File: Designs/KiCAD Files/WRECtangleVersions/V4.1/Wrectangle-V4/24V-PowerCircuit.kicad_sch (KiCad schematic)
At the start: 26 parts, among them M1-24V1 60V, M2-24V1 40V, U7 TPS43060RTER

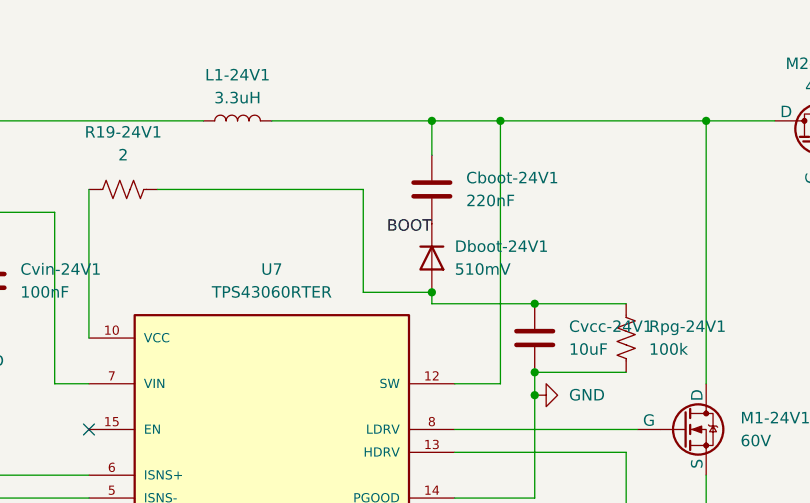
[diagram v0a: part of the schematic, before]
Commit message: Update 24V-PowerCircuit.kicad_sch
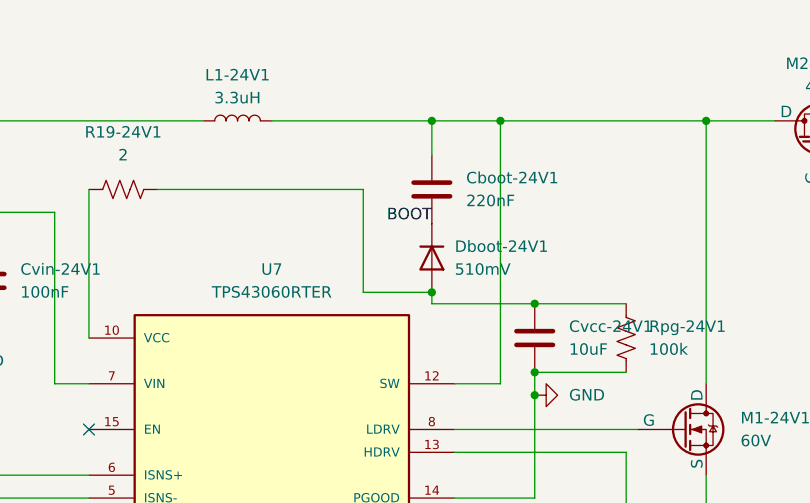
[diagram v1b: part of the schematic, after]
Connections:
- net BOOT: now also Cboot-24V1.1, Dboot-24V1.1 (K)
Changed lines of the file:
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@@
 	)
 	(label "BOOT"
-		(at 181.61 58.42 180)
+		(at 181.61 57.15 180)
 		(effects
 			(font

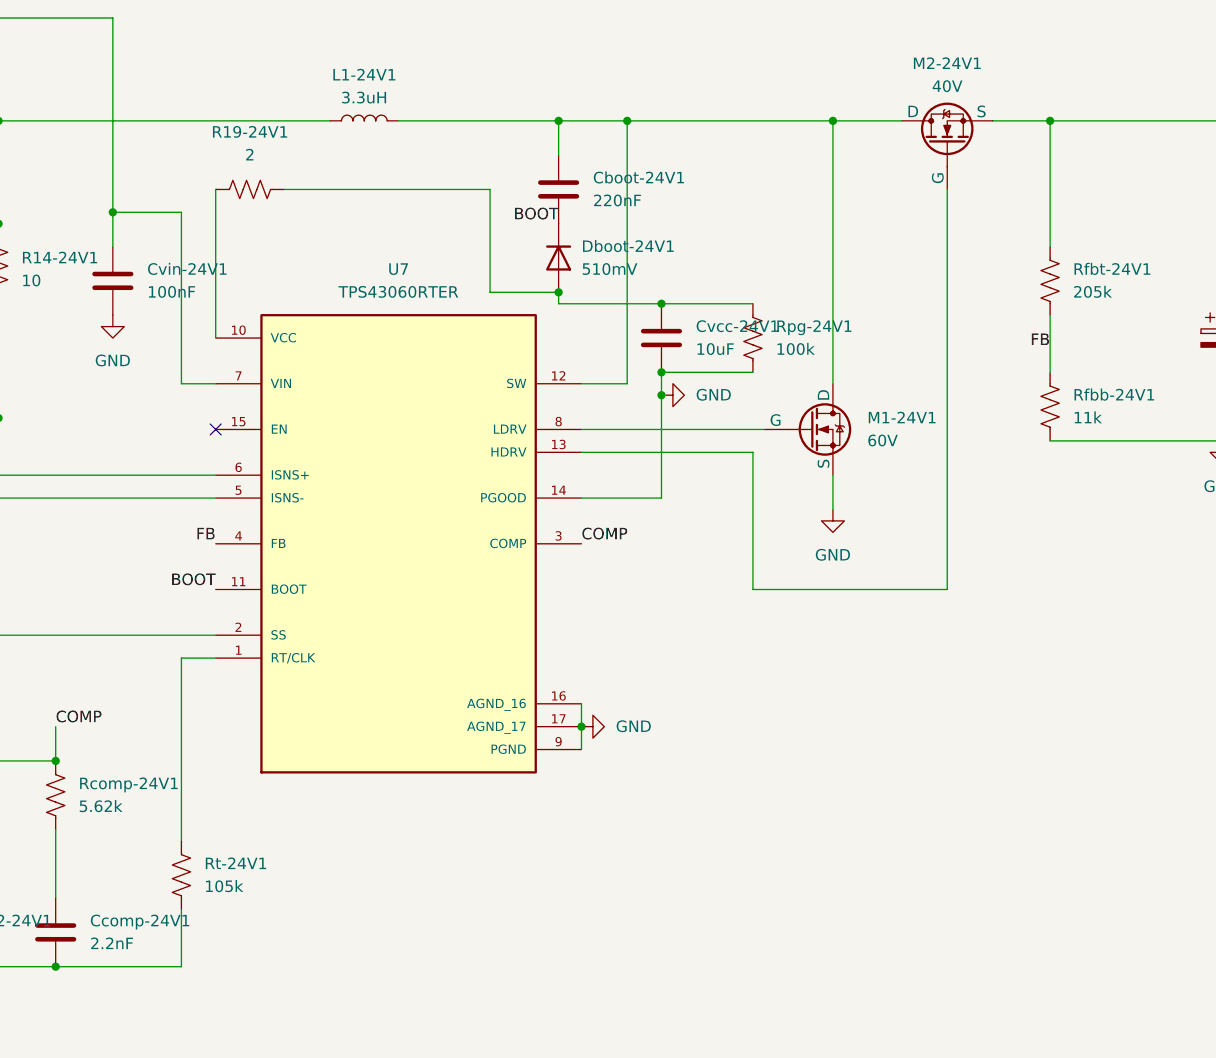
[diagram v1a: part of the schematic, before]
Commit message: Update some schematics (1x)
2-20-26 fixed (#1)
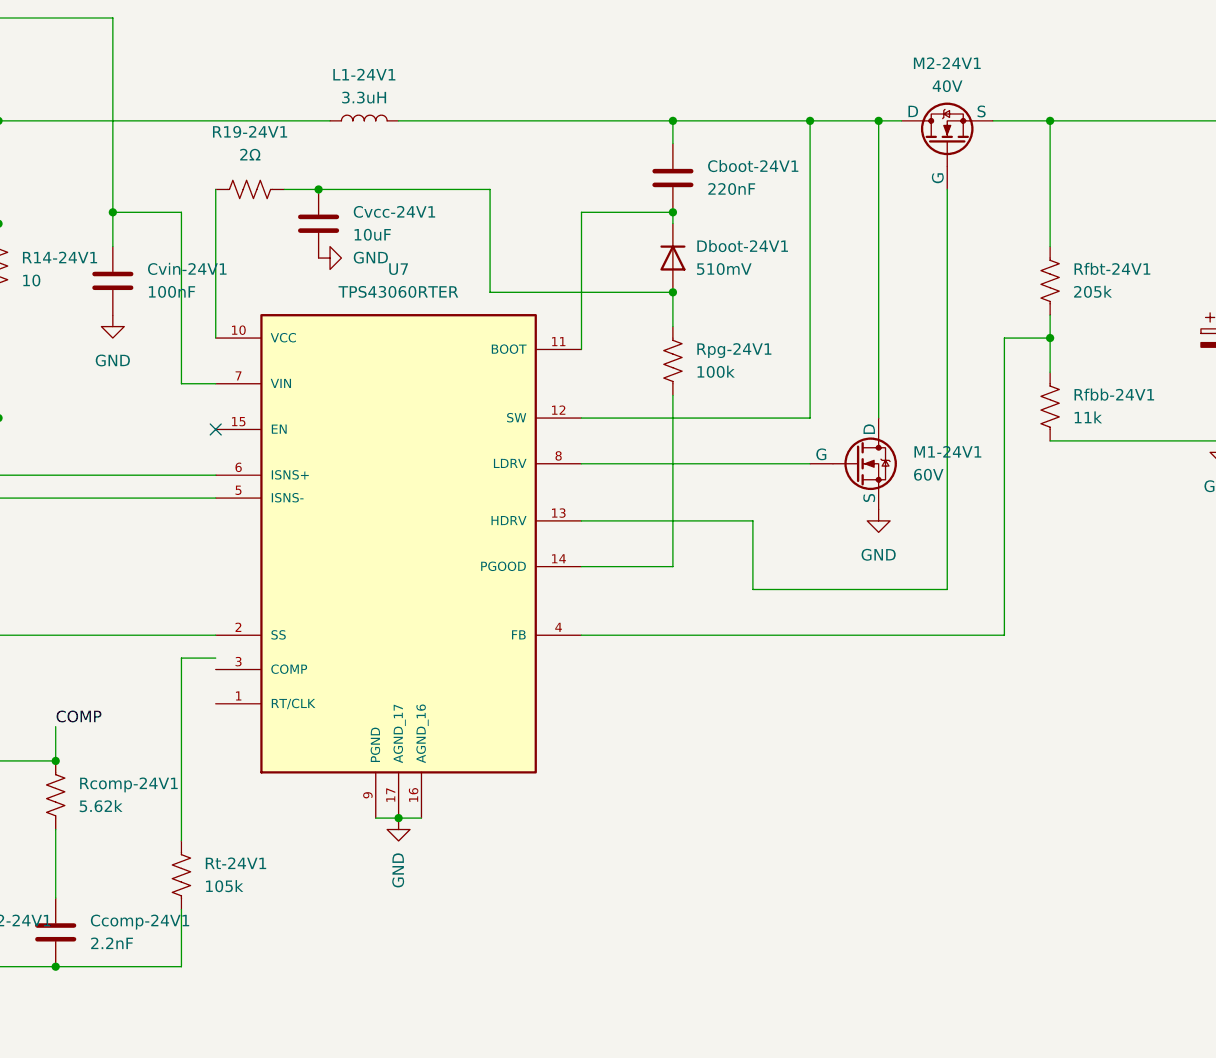
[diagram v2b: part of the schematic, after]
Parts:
- R19-24V1: value 2 -> 2Ω
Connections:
- net 0: no longer Rpg-24V1.1, U7.14 (PGOOD)
- net COMP: no longer U7.3 (COMP)
- net at Rt-24V1.1: no longer U7.1 (RT/CLK)
- net BOOT: no longer names the net of Cboot-24V1.1, Dboot-24V1.1 (K), U7.11 (BOOT)
- net FB: no longer names the net of Rfbb-24V1.2, Rfbt-24V1.1, U7.4 (FB)
- new net: Rpg-24V1.1, U7.14 (PGOOD)
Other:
- moved on the sheet: Cboot-24V1, Cvcc-24V1, Dboot-24V1, M1-24V1, Rpg-24V1, U7

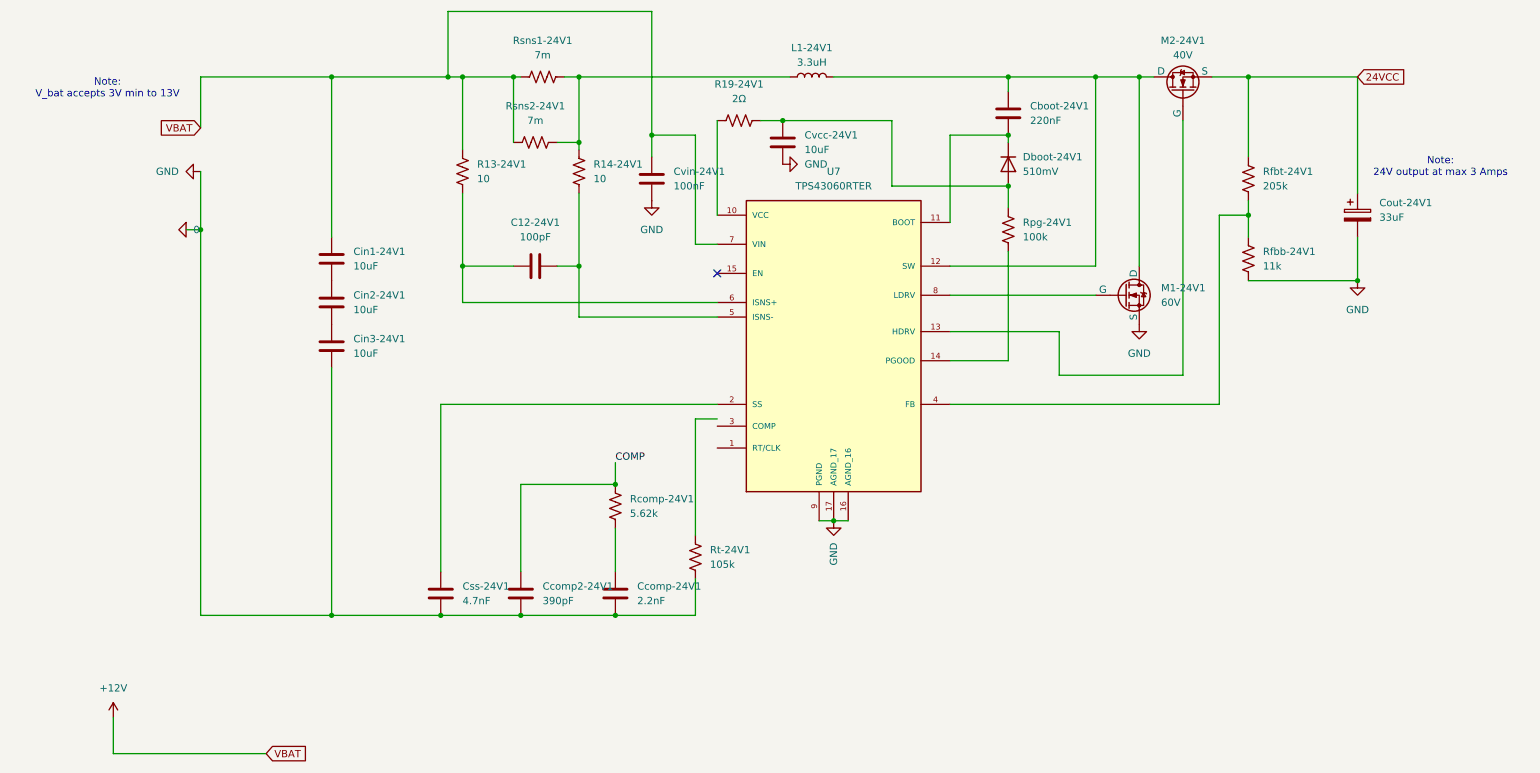
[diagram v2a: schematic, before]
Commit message: Update 24V-PowerCircuit.kicad_sch
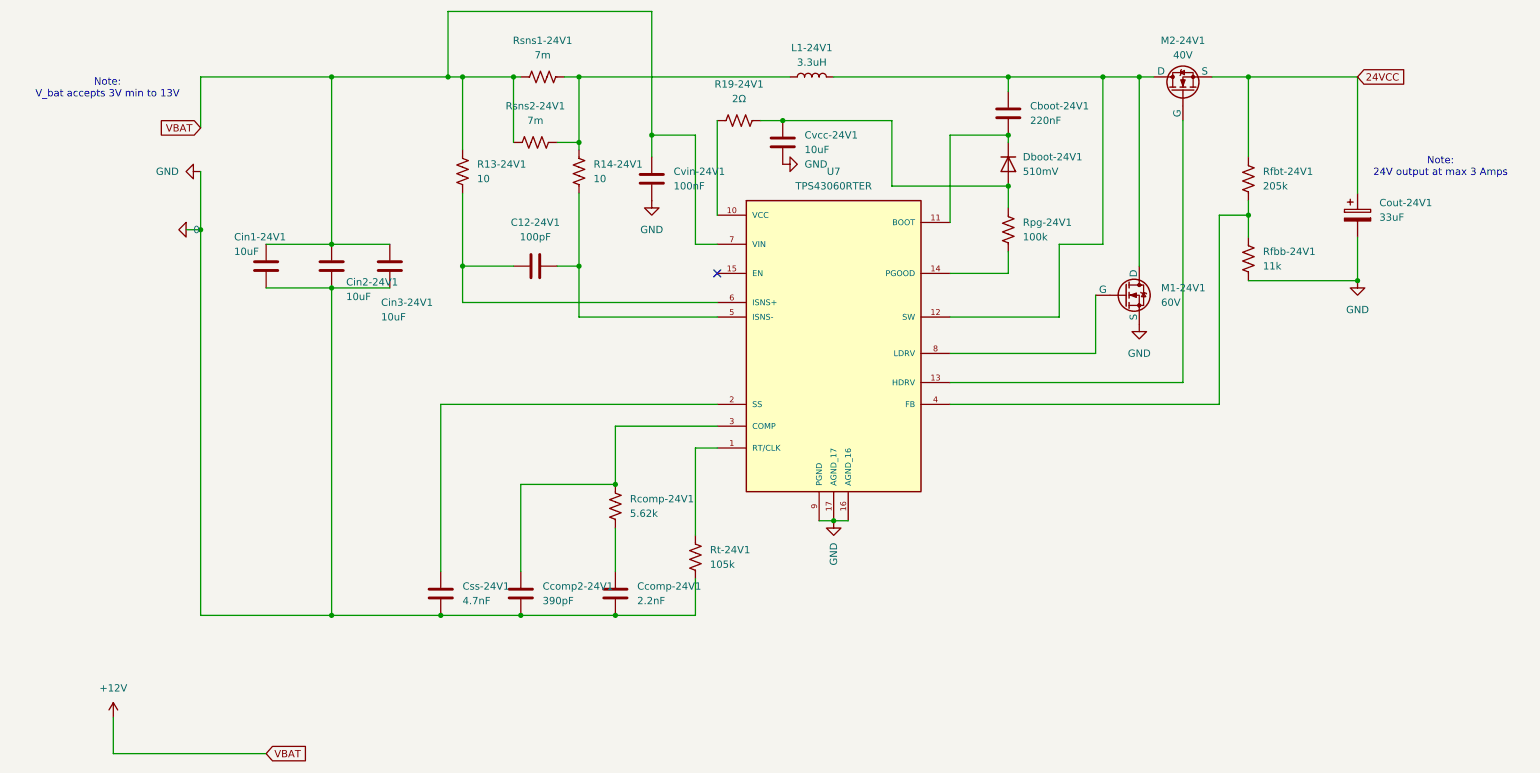
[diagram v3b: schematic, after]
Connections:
- net COMP is gone; now on an unnamed net: Ccomp2-24V1.1, Rcomp-24V1.1
- net +12V: now also Cin2-24V1.1, Cin3-24V1.1
- net 0: now also Cin1-24V1.2, Cin2-24V1.2
- net at Rt-24V1.1: now also U7.1 (RT/CLK)
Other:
- moved on the sheet: Cin1-24V1, Cin2-24V1, Cin3-24V1
